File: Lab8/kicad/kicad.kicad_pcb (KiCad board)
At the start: 2 copper layers, 50.8 x 34.3 mm, 4 parts, among them J1 TI_BOOSTER_40_J1, J2 TI_BOOSTER_40_J2, J3 TI_BOOSTER_40_J3, J4 TI_BOOSTER_40_J4

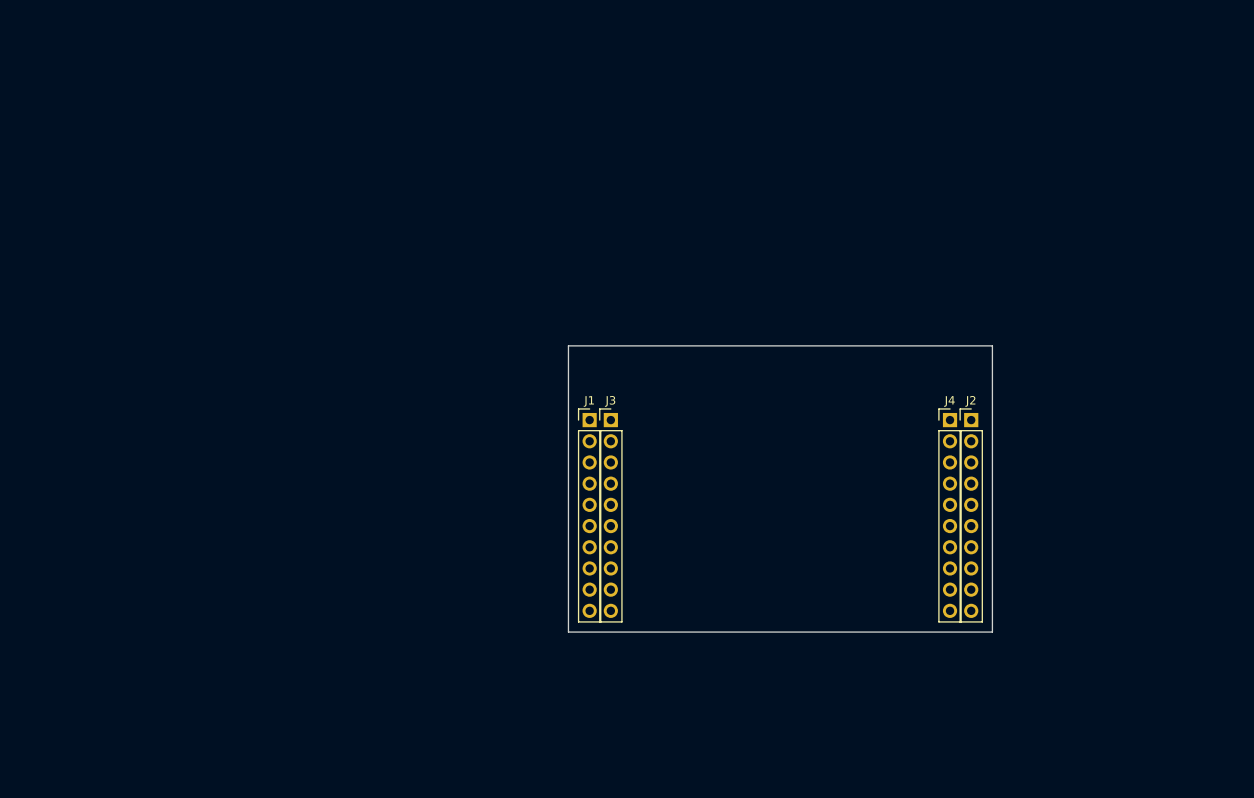
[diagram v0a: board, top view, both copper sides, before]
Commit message: added macros
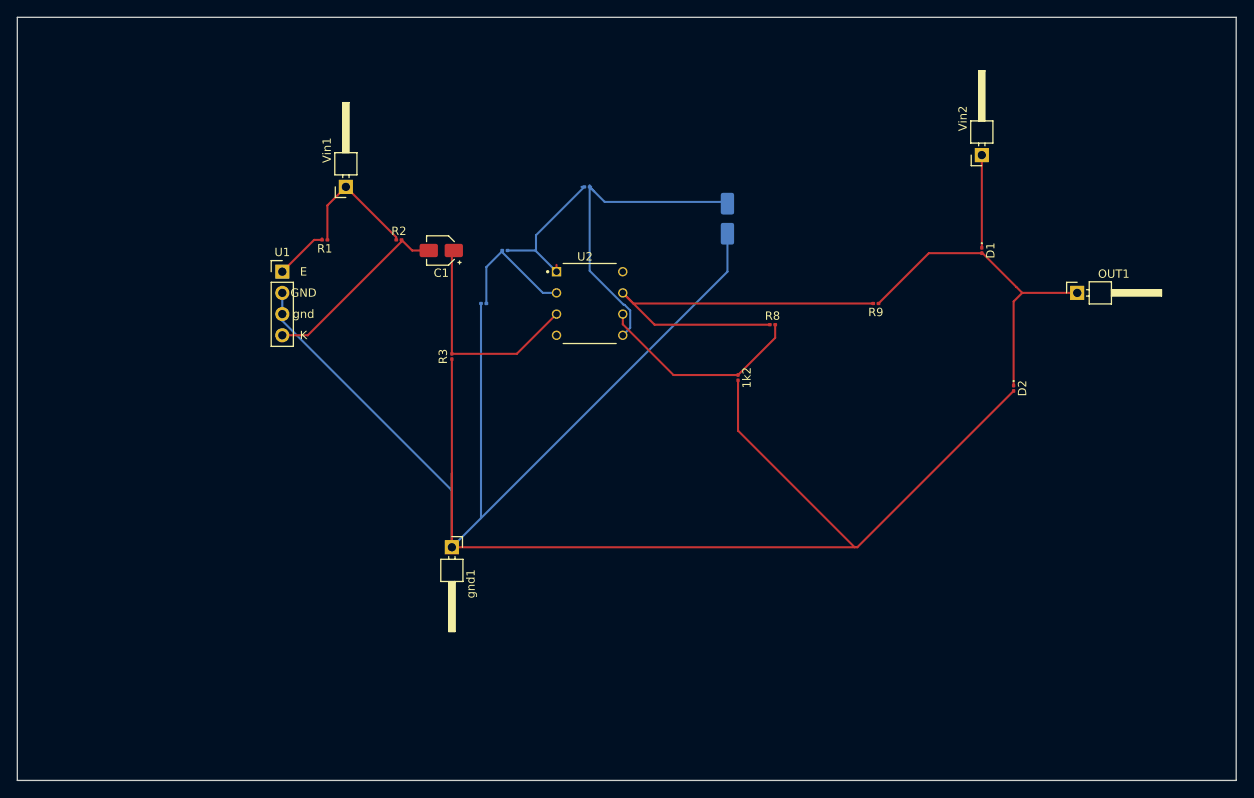
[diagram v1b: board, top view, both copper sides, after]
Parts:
- removed J1: TI_BOOSTER_40_J1, Connector_PinHeader_2.54mm:PinHeader_1x10_P2.54mm_Vertical
- removed J2: TI_BOOSTER_40_J2, Connector_PinHeader_2.54mm:PinHeader_1x10_P2.54mm_Vertical
- removed J3: TI_BOOSTER_40_J3, Connector_PinHeader_2.54mm:PinHeader_1x10_P2.54mm_Vertical
- removed J4: TI_BOOSTER_40_J4, Connector_PinHeader_2.54mm:PinHeader_1x10_P2.54mm_Vertical
- added 1k2: R7, Resistor_SMD:R_0201_0603Metric, F.Cu at (203.2, 116.8)
- added C1: 97.3uf, Capacitor_SMD:CP_Elec_3x5.4, F.Cu at (167.6, 101.6)
- added C2: 97.3uf, Capacitor_SMD:CP_Elec_4x3, B.Cu at (201.9, 97.8)
- added D1: DIODE, Diode_SMD:D_0201_0603Metric, F.Cu at (232.4, 101.6)
- added D2: DIODE, Diode_SMD:D_0201_0603Metric, F.Cu at (236.2, 118.1)
- added OUT1: Conn_01x01_Male, Connector_PinHeader_2.54mm:PinHeader_1x01_P2.54mm_Horizontal, F.Cu at (243.8, 106.7)
- added R1: 82.5, Resistor_SMD:R_0201_0603Metric, F.Cu at (153.7, 100.3)
- added R2: 10k, Resistor_SMD:R_0201_0603Metric, F.Cu at (162.6, 100.3)
- added R3: 680k, Resistor_SMD:R_0201_0603Metric, F.Cu at (168.9, 114.3)
- added R5: 20k, Resistor_SMD:R_0201_0603Metric, B.Cu at (175.3, 101.6)
- added R6: 842k, Resistor_SMD:R_0201_0603Metric, B.Cu at (185.1, 94.0)
- added R8: 15k, Resistor_SMD:R_0201_0603Metric, F.Cu at (207.3, 110.5)
- added R9: 100, Resistor_SMD:R_0201_0603Metric, F.Cu at (219.7, 108.0)
- added U1: OPB745, Connector_PinHeader_2.54mm:PinHeader_1x04_P2.54mm_Vertical, F.Cu at (148.6, 104.1)
- added U2: TLC277, TLC277CP:DIP794W45P254L959H508Q8, F.Cu at (185.4, 108.0)
- added Vin1: Conn_01x01_Male, Connector_PinHeader_2.54mm:PinHeader_1x01_P2.54mm_Horizontal, F.Cu at (156.2, 94.0)
- added Vin2: Conn_01x01_Male, Connector_PinHeader_2.54mm:PinHeader_1x01_P2.54mm_Horizontal, F.Cu at (232.4, 90.2)
- added gnd1: Conn_01x01_Male, Connector_PinHeader_2.54mm:PinHeader_1x01_P2.54mm_Horizontal, F.Cu at (168.9, 137.2)
- added r4: 1k, Resistor_SMD:R_0201_0603Metric, B.Cu at (172.7, 108.0)
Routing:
- net Net-(1k2-Pad2): track 0.00 -> 257.0 mm
- net Net-(R8-Pad1): track 0.00 -> 49.7 mm
- net Net-(D1-Pad2): track 0.00 -> 39.9 mm
- net Net-(C2-Pad1): track 0.00 -> 38.6 mm
- net Net-(C1-Pad1): track 0.00 -> 27.0 mm
- net Net-(1k2-Pad1): track 0.00 -> 25.4 mm
- net Net-(C1-Pad2): track 0.00 -> 22.9 mm
- net Net-(R5-Pad1): track 0.00 -> 18.2 mm
- net Net-(R1-Pad1): track 0.00 -> 16.1 mm
- net Net-(R5-Pad2): track 0.00 -> 15.9 mm
- net Net-(D1-Pad1): track 0.00 -> 11.1 mm
- net Net-(R1-Pad2): track 0.00 -> 6.53 mm
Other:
- board size 50.8 x 34.3 mm -> 146 x 91.4 mm
- copper layers 2 -> 32
- net class Default: clearance 0.254 -> 0.2; trace_width 0.254 -> 0.25; via_dia 0.889 -> 0.8; via_drill 0.635 -> 0.4
- rule trace_clearance: 0.254 -> 0.2
- rule trace_min: 0.254 -> 0.2
- rule via_min_drill: 0.508 -> 0.3
- rule via_min_size: 0.889 -> 0.4
- board text added: "E"
- board text added: "GND"
- board text added: "K"
- board text added: "gnd"
